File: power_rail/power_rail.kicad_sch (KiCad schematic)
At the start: 14 parts, among them J1 Conn_01x06, J2 Conn_02x08_Row_Letter_Last, J3 Conn_02x08_Row_Letter_Last, J4 Conn_02x08_Row_Letter_Last, J5 Conn_02x08_Row_Letter_Last, J6 Conn_02x08_Row_Letter_Last, J7 Conn_02x08_Row_Letter_Last, J8 Conn_01x06

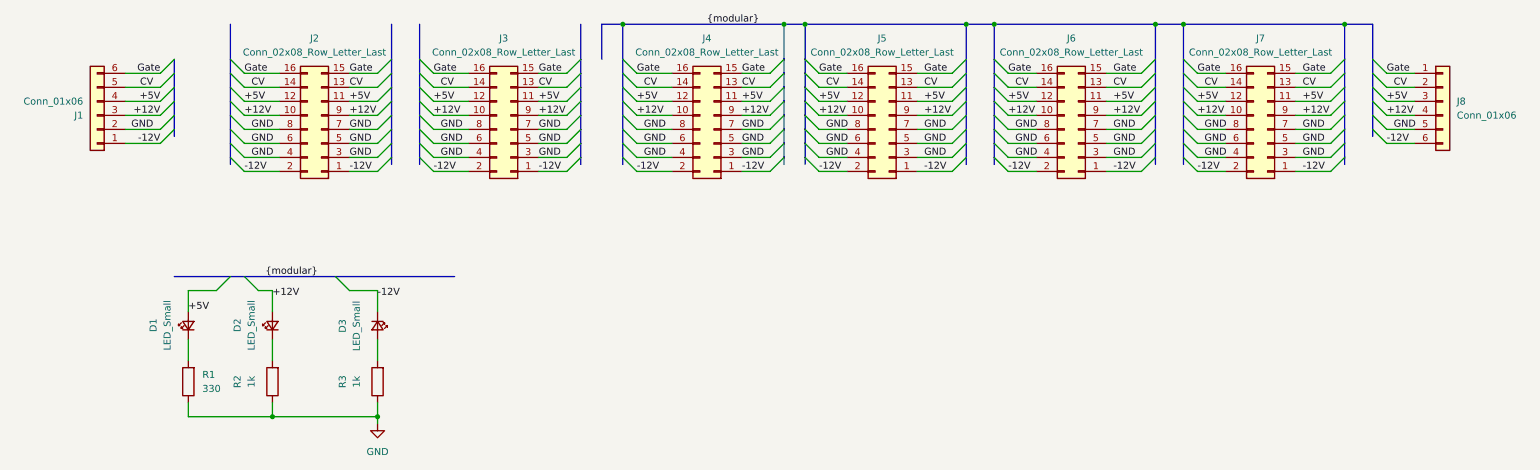
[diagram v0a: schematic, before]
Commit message: VCA v. 2.0
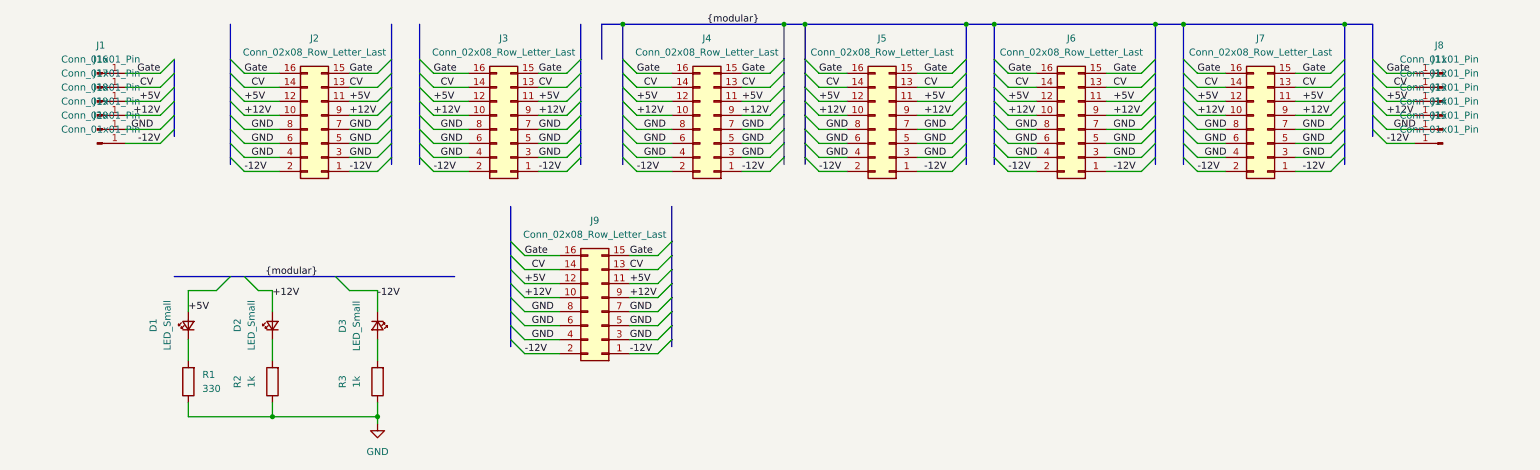
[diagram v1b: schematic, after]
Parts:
- removed J1, J8: Conn_01x06, Connector_Wire:SolderWire-0.75sqmm_1x06_P4.8mm_D1.25mm_OD2.3mm, symbol Connector_Generic:Conn_01x06
- added J1, J11, J12, J13, J14, J15, J16, J17, J18, J19, J20, J8: Conn_01x01_Pin, power_rail_elements:Blade_3866B.68, symbol Connector:Conn_01x01_Pin
- added J9: Conn_02x08_Row_Letter_Last, Connector_IDC:IDC-Header_2x08_P2.54mm_Vertical, symbol Connector_Generic:Conn_02x08_Odd_Even
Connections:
- net +12V: now also J13.1 (Pin_1), J18.1 (Pin_1), J9.10 (Pin_10), J9.9 (Pin_9)
- net +5V: now also J12.1 (Pin_1), J17.1 (Pin_1), J9.11 (Pin_11), J9.12 (Pin_12)
- net -12V: now also J15.1 (Pin_1), J20.1 (Pin_1), J9.1 (Pin_1), J9.2 (Pin_2)
- net CV: now also J11.1 (Pin_1), J16.1 (Pin_1), J9.13 (Pin_13), J9.14 (Pin_14)
- net GND: now also J14.1 (Pin_1), J19.1 (Pin_1), J9.3 (Pin_3), J9.4 (Pin_4), J9.5 (Pin_5), J9.6 (Pin_6), J9.7 (Pin_7), J9.8 (Pin_8)
- net Gate: now also J1.1 (Pin_1), J8.1 (Pin_1), J9.15 (Pin_15), J9.16 (Pin_16)
